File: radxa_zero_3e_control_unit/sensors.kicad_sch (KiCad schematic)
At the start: 17 parts, among them J15 Weight, Q1 BC807, U3 HX711

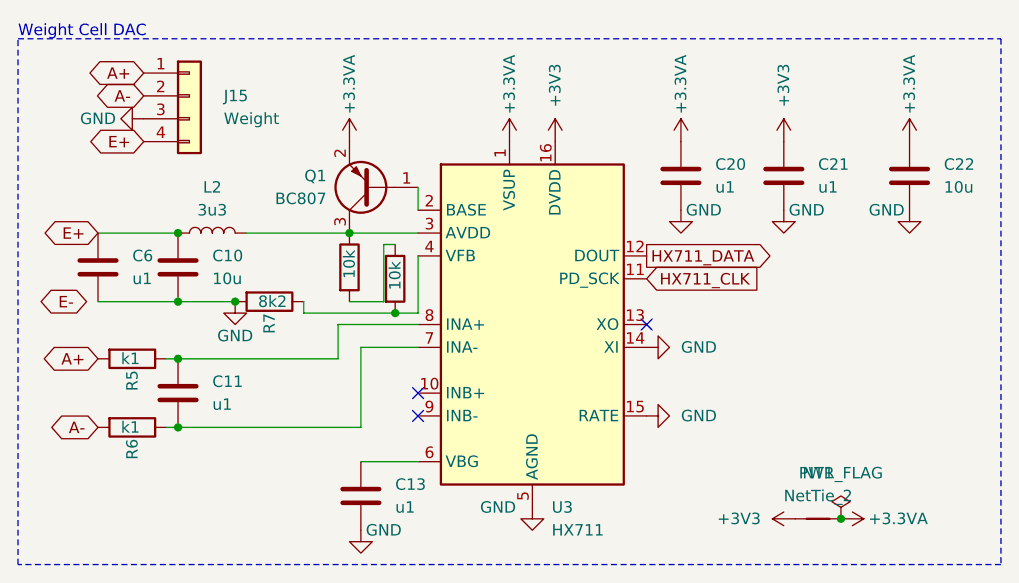
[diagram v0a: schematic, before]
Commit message: Udated control unit pcb
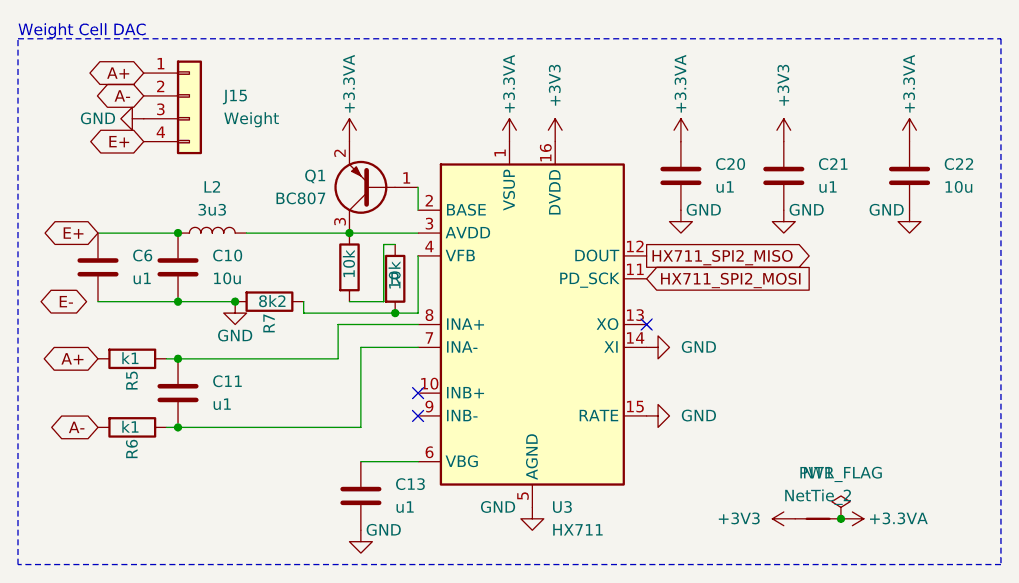
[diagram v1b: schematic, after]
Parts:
- C11, C13, C20, C21, C6: footprint Capacitor_SMD:C_0201_0603Metric -> Capacitor_SMD:C_0402_1005Metric
- J15: footprint liebler_CONN:JST_XH_S4B-XH-A-1_1x04_P2.50mm_Horizontal_SmallerCourtyard -> liebler_CONN:JST_XH_B4B-XH-A_1x04_P2.50mm_Vertical_smaller
- R11, R8: footprint Resistor_SMD:R_0201_0603Metric -> Resistor_SMD:R_0402_1005Metric
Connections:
- net HX711_CLK renamed HX711_SPI2_MOSI
- net HX711_DATA renamed HX711_SPI2_MISO
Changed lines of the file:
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@@
+		)
+	)
+	(global_label "HX711_SPI2_MISO"
+		(shape output)
+		(at 83.82 39.37 0)
+		(fields_autoplaced yes)
+		(effects
+			(font
+				(size 1.27 1.27)
+			)
+			(justify left)
+		)
+		(property "Intersheetrefs" "${INTERSHEET_REFS}"
+			(at 103.7989 39.37 0)
+			(effects
+				(font
+					(size 1.27 1.27)
+				)
+				(justify left)
+				(hide yes)
+			)
 		)
 	)
@@
 		)
 	)
-	(global_label "HX711_DATA"
-		(shape output)
-		(at 83.82 39.37 0)
-		(fields_autoplaced yes)
-		(effects
-			(font
-				(size 1.27 1.27)
-			)
-			(justify left)
-		)
-		(property "Intersheetrefs" "${INTERSHEET_REFS}"
-			(at 98.3561 39.37 0)
-			(effects
-				(font
-					(size 1.27 1.27)
-				)
-				(justify left)
-				(hide yes)
-			)
-		)
-	)
-	(global_label "HX711_CLK"
+	(global_label "HX711_SPI2_MOSI"
 		(shape input)
 		(at 83.82 41.91 0)
@@
 		)
 		(property "Intersheetrefs" "${INTERSHEET_REFS}"
-			(at 97.5094 41.91 0)
+			(at 103.7989 41.91 0)
 			(effects
 				(font
@@
 			)
 		)
-		(property "Footprint" "Capacitor_SMD:C_0201_0603Metric"
+		(property "Footprint" "Capacitor_SMD:C_0402_1005Metric"
 			(at 23.8252 44.45 0)
 			(effects
@@
 			)
 		)
-		(property "Footprint" "Capacitor_SMD:C_0201_0603Metric"
+		(property "Footprint" "Capacitor_SMD:C_0402_1005Metric"
 			(at 53.0352 69.85 0)
 			(effects
@@
 			)
 		)
-		(property "Footprint" "Capacitor_SMD:C_0201_0603Metric"
+		(property "Footprint" "Capacitor_SMD:C_0402_1005Metric"
 			(at 100.0252 34.29 0)
 			(effects
@@
 			)
 		)
-		(property "Footprint" "liebler_CONN:JST_XH_S4B-XH-A-1_1x04_P2.50mm_Horizontal_SmallerCourtyard"
+		(property "Footprint" "liebler_CONN:JST_XH_B4B-XH-A_1x04_P2.50mm_Vertical_smaller"
 			(at 33.02 21.59 0)
 			(effects
@@
 			)
 		)
-		(property "Footprint" "Resistor_SMD:R_0201_0603Metric"
+		(property "Footprint" "Resistor_SMD:R_0402_1005Metric"
 			(at 54.102 41.91 90)
 			(effects
@@
 				)
 				(hide yes)
+			)
+		)
+		(property "Sim.Device" "R"
+			(at 55.88 41.91 0)
+			(effects
+				(font
+					(size 1.27 1.27)
+				)
+			)
+		)
+		(property "Sim.Pins" ""
+			(at 55.88 41.91 0)
+			(effects
+				(font
+					(size 1.27 1.27)
+				)
 			)
 		)
@@
 			)
 		)
-		(property "Footprint" "Capacitor_SMD:C_0201_0603Metric"
+		(property "Footprint" "Capacitor_SMD:C_0402_1005Metric"
 			(at 32.7152 58.42 0)
 			(effects
@@
 			)
 		)
-		(property "Footprint" "Capacitor_SMD:C_0201_0603Metric"
+		(property "Footprint" "Capacitor_SMD:C_0402_1005Metric"
 			(at 88.5952 34.29 0)
 			(effects
@@
 			)
 		)
-		(property "Footprint" "Resistor_SMD:R_0201_0603Metric"
+		(property "Footprint" "Resistor_SMD:R_0402_1005Metric"
 			(at 49.022 40.64 90)
 			(effects
